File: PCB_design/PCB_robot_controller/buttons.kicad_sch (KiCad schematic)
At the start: 6 parts, among them SW1 SW_SPDT, SW2 SW_SPDT, SW3 SW_SPDT

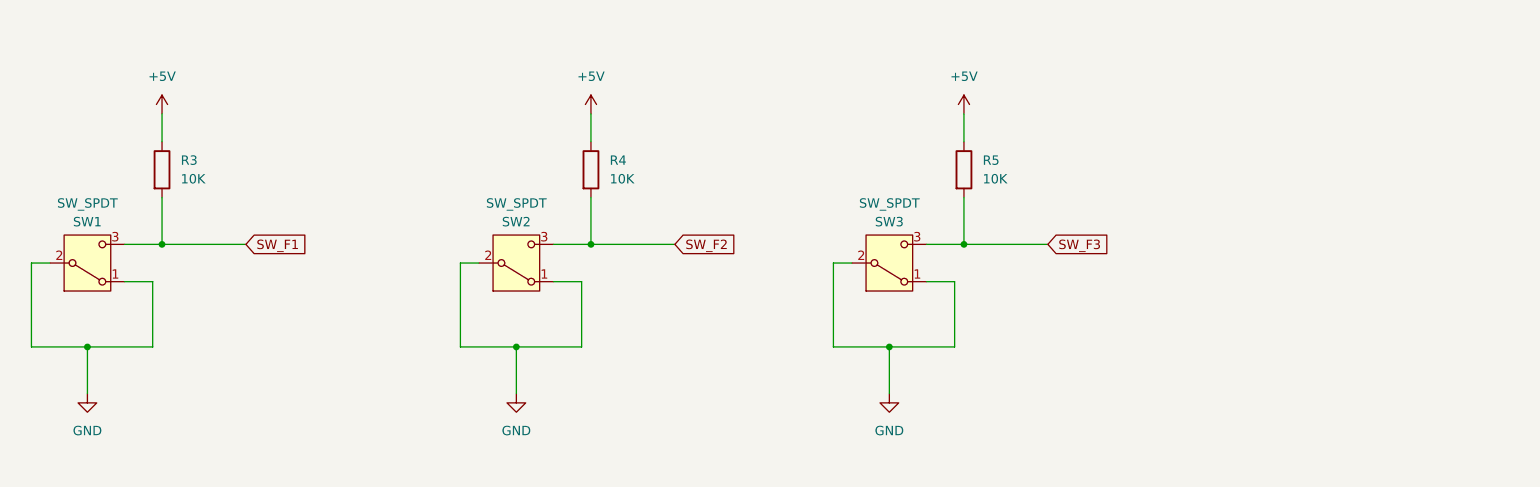
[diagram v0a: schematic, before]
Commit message: pcb to production
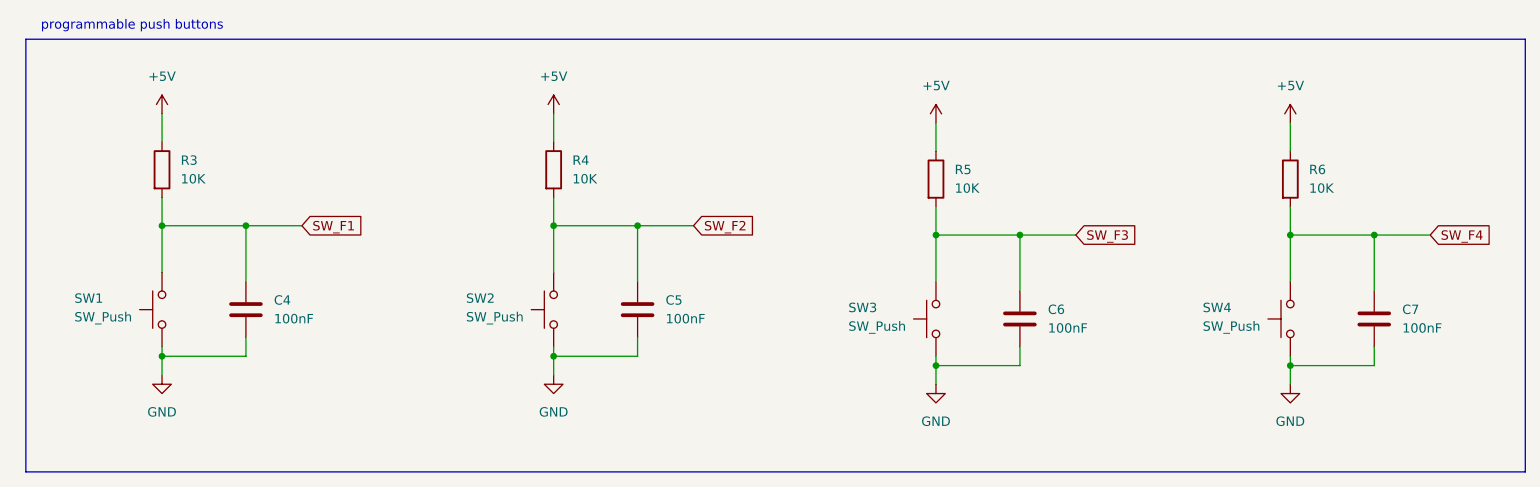
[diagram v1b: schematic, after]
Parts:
- removed SW1, SW2, SW3: SW_SPDT, symbol Switch:SW_SPDT
- added C4, C5, C6, C7: 100nF, Capacitor_SMD:C_0805_2012Metric, symbol Device:C
- added R6: 10K, Resistor_SMD:R_0805_2012Metric, symbol Device:R
- added SW1, SW2, SW3, SW4: SW_Push, Button_Switch_THT:SW_PUSH_6mm_H5mm, symbol Switch:SW_Push
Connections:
- net +5V: now also R6.1
- net GND: now also C4.2, C5.2, C6.2, C7.2, SW1.1, SW2.1, SW3.1, SW4.1
- net SW_F1: now also C4.1, SW1.2
- net SW_F2: now also C5.1, SW2.2
- net SW_F3: now also C6.1, SW3.2
- new net SW_F4: C7.1, R6.2, SW4.2
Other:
- note added: "programmable push buttons"
